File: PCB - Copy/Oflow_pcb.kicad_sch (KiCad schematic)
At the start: 2 parts, among them U1 node

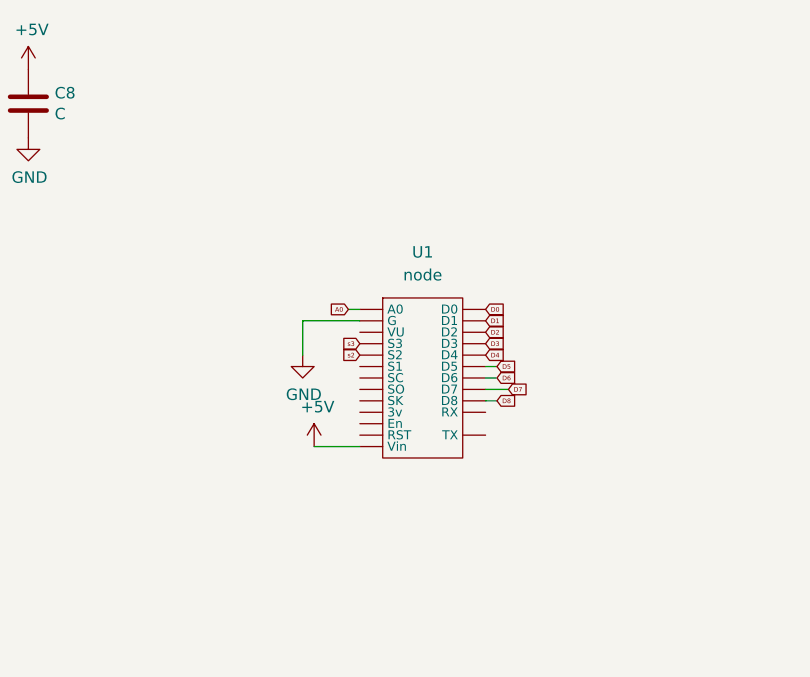
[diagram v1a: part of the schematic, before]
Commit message: added nod
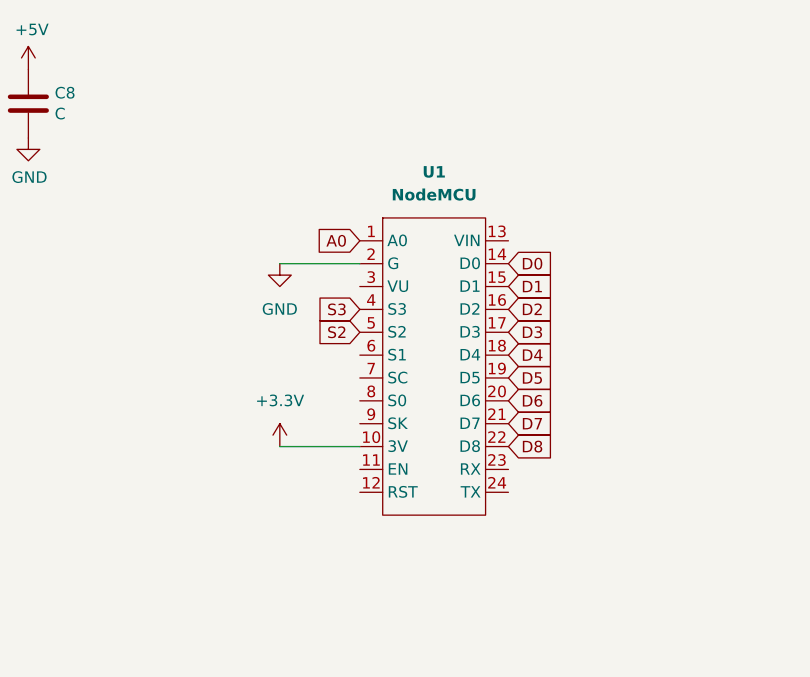
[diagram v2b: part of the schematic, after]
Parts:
- removed U1: node, SHAHIDABDULLA:espnode, symbol SHA:node
- added U1: NodeMCU, NodeMCU:NODE V1, symbol New_Library:NodeMCU
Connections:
- net A0: now also U1.1 (A0)
- net D0: now also U1.14 (D0)
- net D1: now also U1.15 (D1)
- net D2: now also U1.16 (D2)
- net D3: now also U1.17 (D3)
- net D4: now also U1.18 (D4)
- net D5: now also U1.19 (D5)
- net D6: now also U1.20 (D6)
- net D7: now also U1.21 (D7)
- net D8: now also U1.22 (D8)
- net GND: now also U1.2 (G)
- new net +3.3V: U1.10 (3V)
- new net S2: U1.5 (S2)
- new net S3: U1.4 (S3)
